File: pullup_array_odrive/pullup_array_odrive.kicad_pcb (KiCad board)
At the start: 2 copper layers, 62.2 x 31.7 mm, 29 parts, among them J9 Conn_01x20_Male

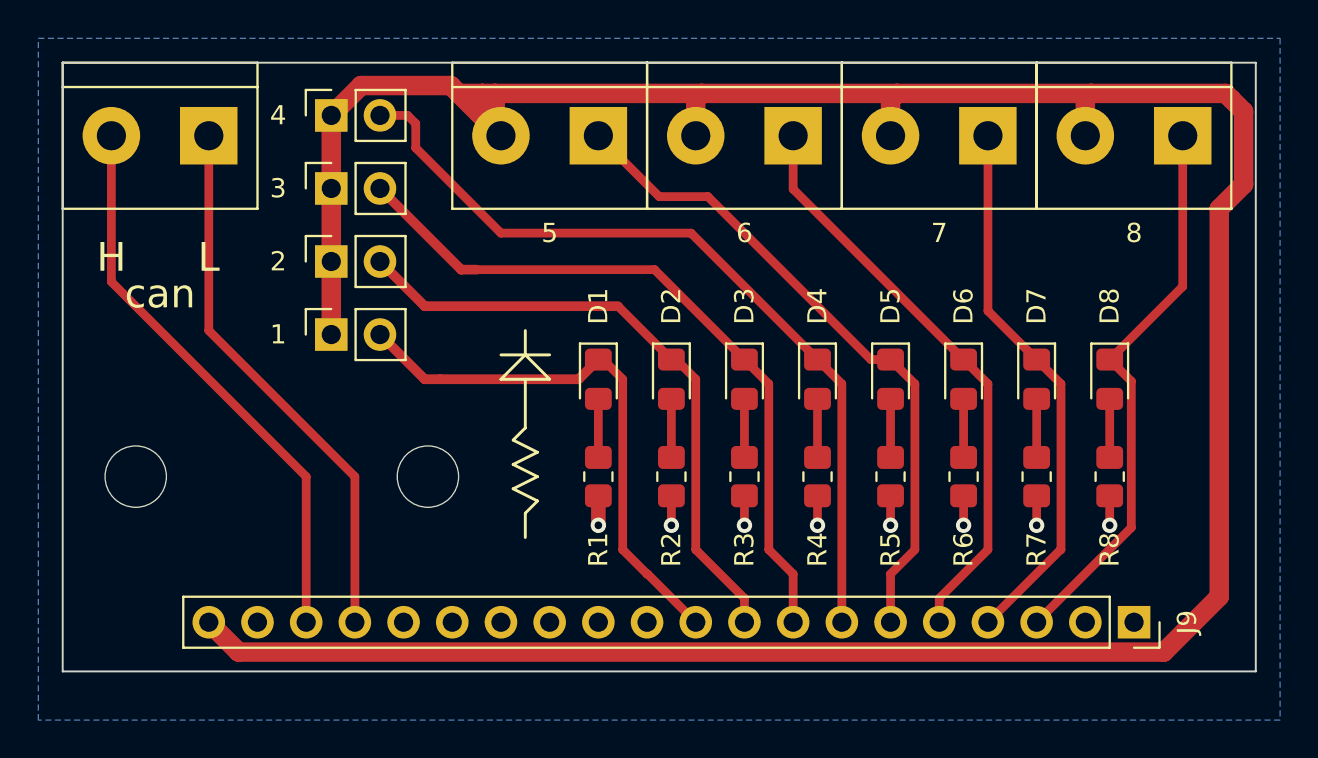
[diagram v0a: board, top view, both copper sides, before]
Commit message: last changes
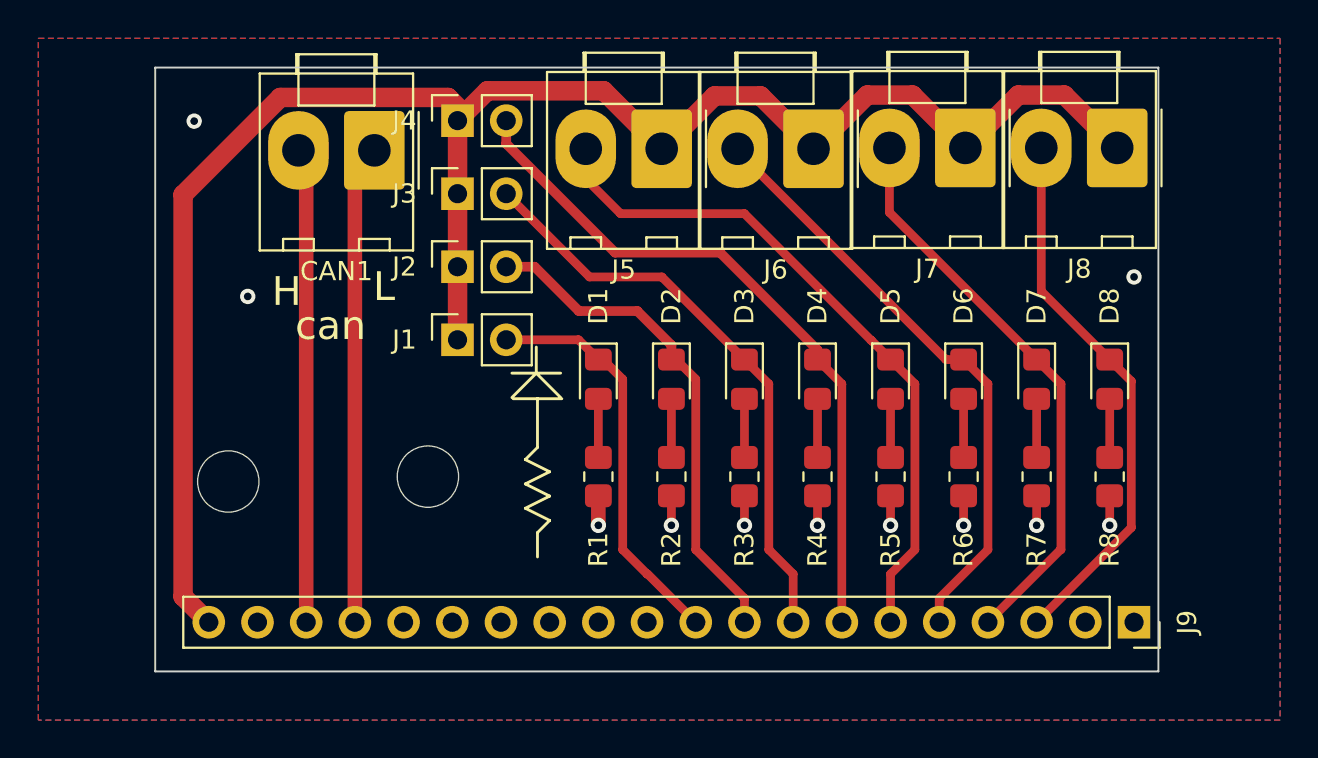
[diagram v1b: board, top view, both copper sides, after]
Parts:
- CAN1: footprint TerminalBlock:TerminalBlock_bornier-2_P5.08mm -> Connector_Molex:Molex_KK-396_A-41791-0002_1x02_P3.96mm_Vertical
- J5: renamed from 5; footprint TerminalBlock:TerminalBlock_bornier-2_P5.08mm -> Connector_Molex:Molex_KK-396_A-41791-0002_1x02_P3.96mm_Vertical
- J6: renamed from 6; footprint TerminalBlock:TerminalBlock_bornier-2_P5.08mm -> Connector_Molex:Molex_KK-396_A-41791-0002_1x02_P3.96mm_Vertical
- J7: renamed from 7; footprint TerminalBlock:TerminalBlock_bornier-2_P5.08mm -> Connector_Molex:Molex_KK-396_A-41791-0002_1x02_P3.96mm_Vertical
- J8: renamed from 8; footprint TerminalBlock:TerminalBlock_bornier-2_P5.08mm -> Connector_Molex:Molex_KK-396_A-41791-0002_1x02_P3.96mm_Vertical
- moved CAN1 8.67 mm to (111.5, 51.6)
- moved J1 6.59 mm to (115.8, 61.4)
- moved J2 6.59 mm to (115.8, 57.6)
- moved J3 6.59 mm to (115.8, 53.8)
- moved J4 6.59 mm to (115.8, 50.0)
- moved REF** 4.83 mm to (103.9, 68.8)
- moved J8 3.48 mm to (150.3, 51.4)
- moved J5 3.37 mm to (126.5, 51.5)
- moved J7 1.34 mm to (142.3, 51.4)
- moved G*** 1.31 mm to (127.0, 61.7)
- moved J6 1.26 mm to (134.4, 51.5)
- renumbered 1 to J1, 2 to J2, 3 to J3, 4 to J4
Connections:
- J5 pad 1: Net-(D5-Pad1) -> +3V3
- J5 pad 2: +3V3 -> Net-(D5-Pad1)
- J6 pad 1: Net-(D6-Pad1) -> +3V3
- J6 pad 2: +3V3 -> Net-(D6-Pad1)
- J7 pad 1: Net-(D7-Pad1) -> +3V3
- J7 pad 2: +3V3 -> Net-(D7-Pad1)
- J8 pad 1: Net-(D8-Pad1) -> +3V3
- J8 pad 2: +3V3 -> Net-(D8-Pad1)
- J9 pad 16: GND -> unconnected-(J9-Pad16)
- J9 pad 19: GND -> unconnected-(J9-Pad19)
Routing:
- net +3V3: track 156.3 -> 94.6 mm
- net Net-(D1-Pad1): track 28.7 -> 21.2 mm
- net Net-(D3-Pad1): track 37.5 -> 30.8 mm
- net Net-(D4-Pad1): track 43.1 -> 36.6 mm
- net Net-(D2-Pad1): track 32.7 -> 26.5 mm
- net Net-(CAN1-Pad2): track 29.6 -> 24.8 mm
- net Net-(CAN1-Pad1): track 28.5 -> 25.0 mm
- net Net-(D7-Pad1): track 28.5 -> 30.0 mm
- net Net-(D5-Pad1): track 34.8 -> 36.1 mm
- net Net-(D6-Pad1): track 30.6 -> 31.7 mm
- net Net-(D8-Pad1): track 29.5 -> 28.7 mm
- net GND: vias 8 -> 11
- added copper zone on F.Cu, net GND
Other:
- board size 62.2 x 31.7 mm -> 52.3 x 31.5 mm
